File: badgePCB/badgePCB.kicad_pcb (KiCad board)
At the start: 2 copper layers, 81.7 x 39.6 mm, 28 parts, among them SW1 TS-1187A-B-A-B, SW2 TS-1187A-B-A-B, SW3 TS-1187A-B-A-B, U1 XIAO-ESP32-C3-DIP

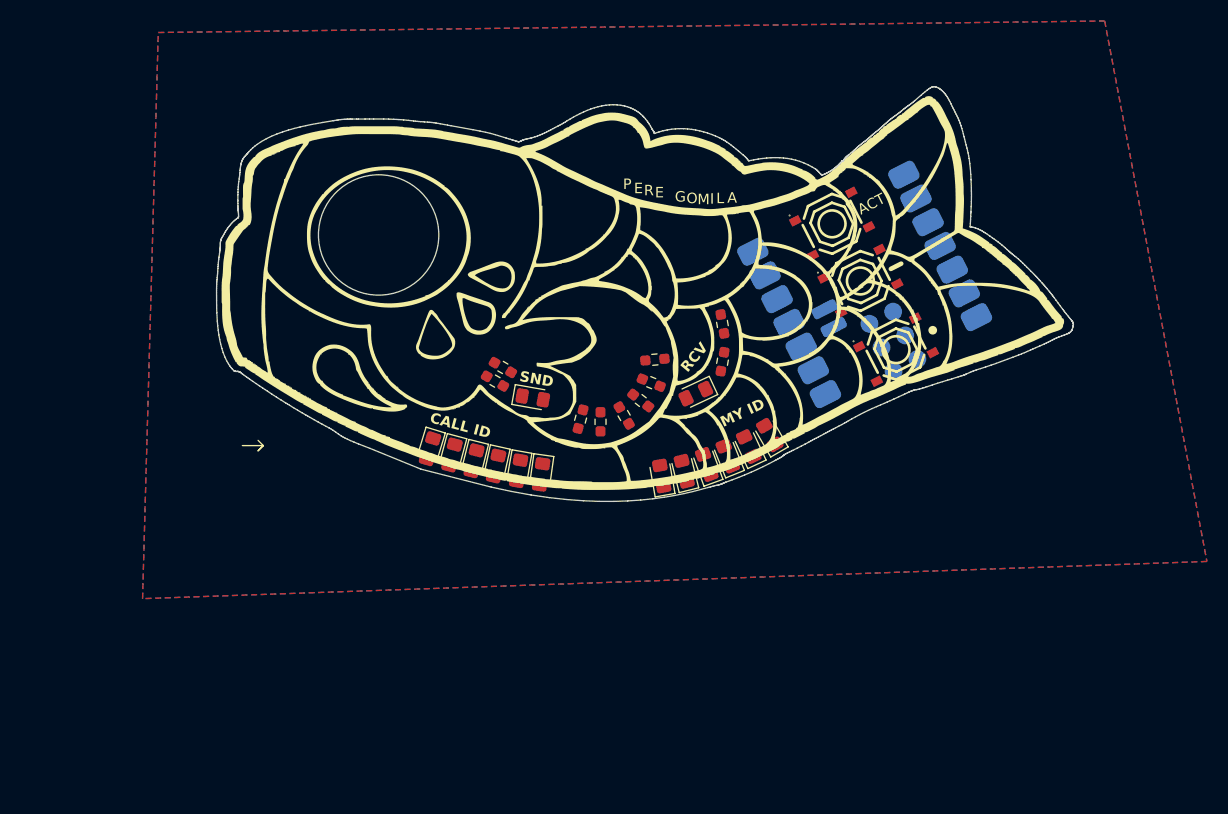
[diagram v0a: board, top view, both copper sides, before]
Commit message: finishPCB
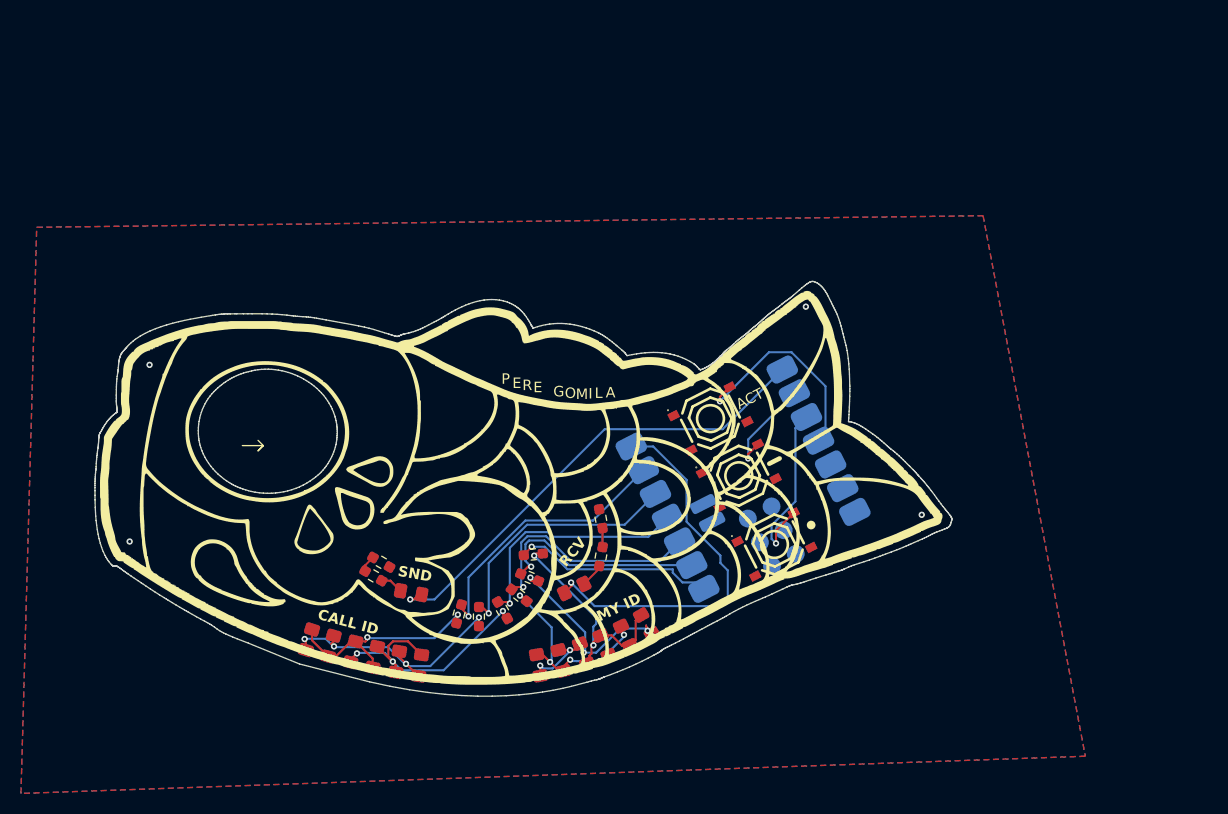
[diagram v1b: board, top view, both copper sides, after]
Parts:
- D1, D10, D11, D12, D13, D14, D2, D3, D4, D5, D6, D7, D8, D9: footprint LED_SMD:LED_0805_2012Metric_Pad1.15x1.40mm_HandSolder -> Extra:LED_0805_2012Metric_Pad1.15x1.40mm_HandSolder
- moved R1 21.9 mm to (63.8, 74.6)
- moved R10 21.9 mm to (71.6, 67.3)
- moved R2 21.9 mm to (64.8, 72.9)
- moved R7 21.9 mm to (71.6, 70.9)
- moved SW3 21.9 mm to (82.1, 57.7)
- moved U1 21.9 mm to (85.1, 63.6)
- moved D14 21.9 mm to (53.5, 74.3)
- moved R5 21.9 mm to (60.0, 76.6)
- moved R6 21.9 mm to (58.1, 76.4)
- moved D13 21.9 mm to (69.1, 73.9)
- moved R3 21.9 mm to (65.2, 70.7)
- moved R4 21.9 mm to (62.2, 76.0)
- moved R8 21.9 mm to (49.9, 72.7)
- moved R9 21.9 mm to (50.7, 71.4)
- moved SW1 21.9 mm to (84.8, 63.2)
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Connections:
- U1 pad 1: MID1 -> MID3
- U1 pad 2: MID2 -> MID1
- U1 pad 3: MID3 -> MID2
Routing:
- net SLED: track 0.00 -> 45.9 mm, vias 0 -> 1
- net RLED: track 0.00 -> 37.0 mm, vias 0 -> 1
- net Net-(D10-A): track 0.00 -> 27.8 mm, vias 0 -> 3
- net Net-(D1-K): track 0.00 -> 26.6 mm, vias 0 -> 5
- net SID3: track 0.00 -> 26.0 mm, vias 0 -> 1
- net Net-(D11-K): track 0.00 -> 25.8 mm, vias 0 -> 4
- net SID2: track 0.00 -> 24.6 mm, vias 0 -> 1
- net SID1: track 0.00 -> 23.1 mm, vias 0 -> 1
- net Net-(D3-K): track 0.00 -> 23.1 mm, vias 0 -> 2
- net MID2: track 0.00 -> 22.7 mm, vias 0 -> 1
- net Net-(D1-A): track 0.00 -> 22.2 mm, vias 0 -> 5
- net Net-(D10-K): track 0.00 -> 21.5 mm, vias 0 -> 2
- net MID1: track 0.00 -> 20.8 mm, vias 0 -> 1
- net Action: track 0.00 -> 20.6 mm, vias 0 -> 1
- net MID3: track 0.00 -> 19.4 mm, vias 0 -> 1
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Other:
- outline, holes or cut-outs redrawn
